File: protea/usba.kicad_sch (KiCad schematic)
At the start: 5 parts, among them J3 676430910, U7 USBLC6-2SC6

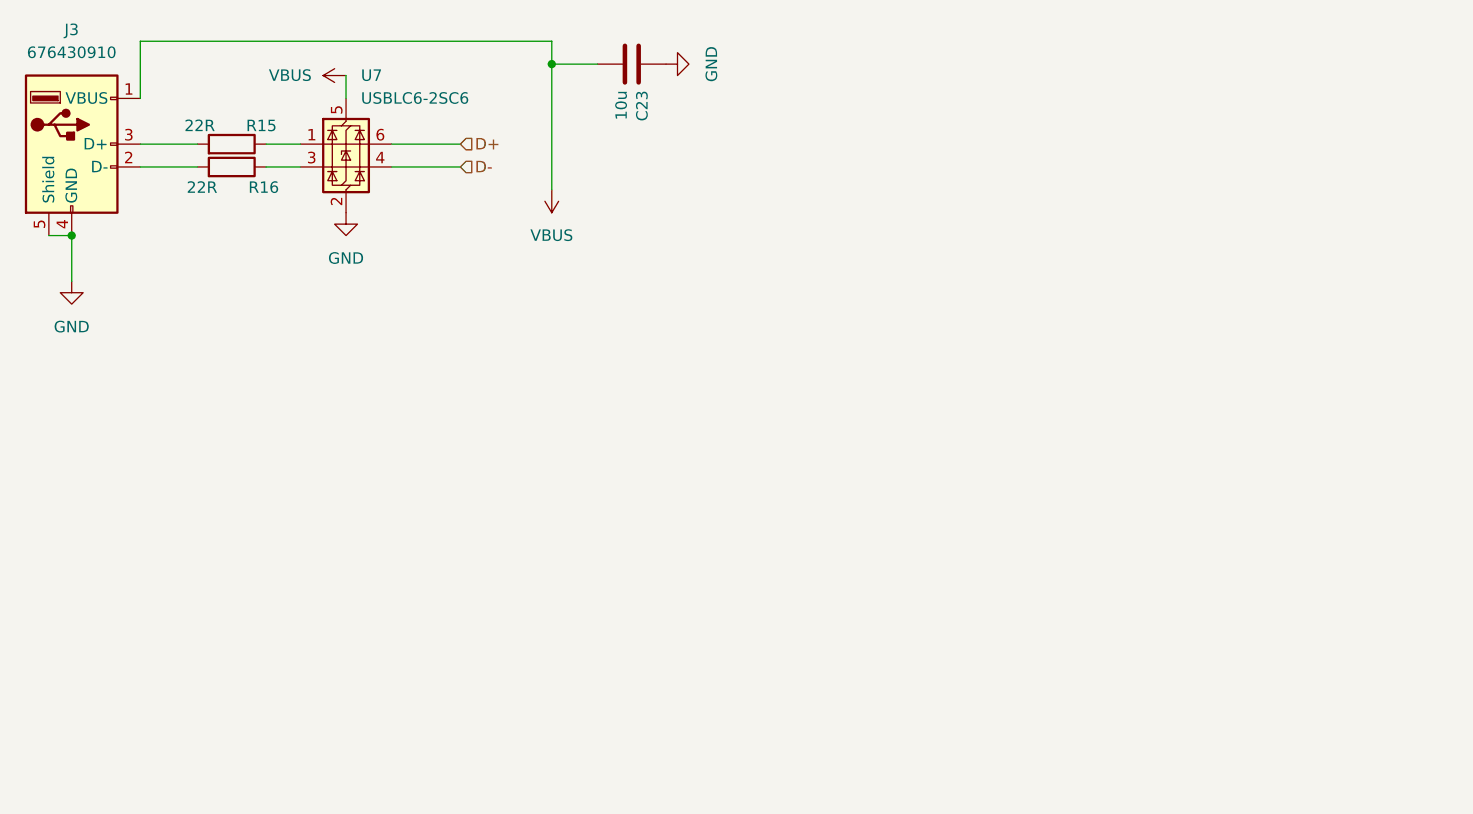
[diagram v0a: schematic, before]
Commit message: Protea HW 2.06
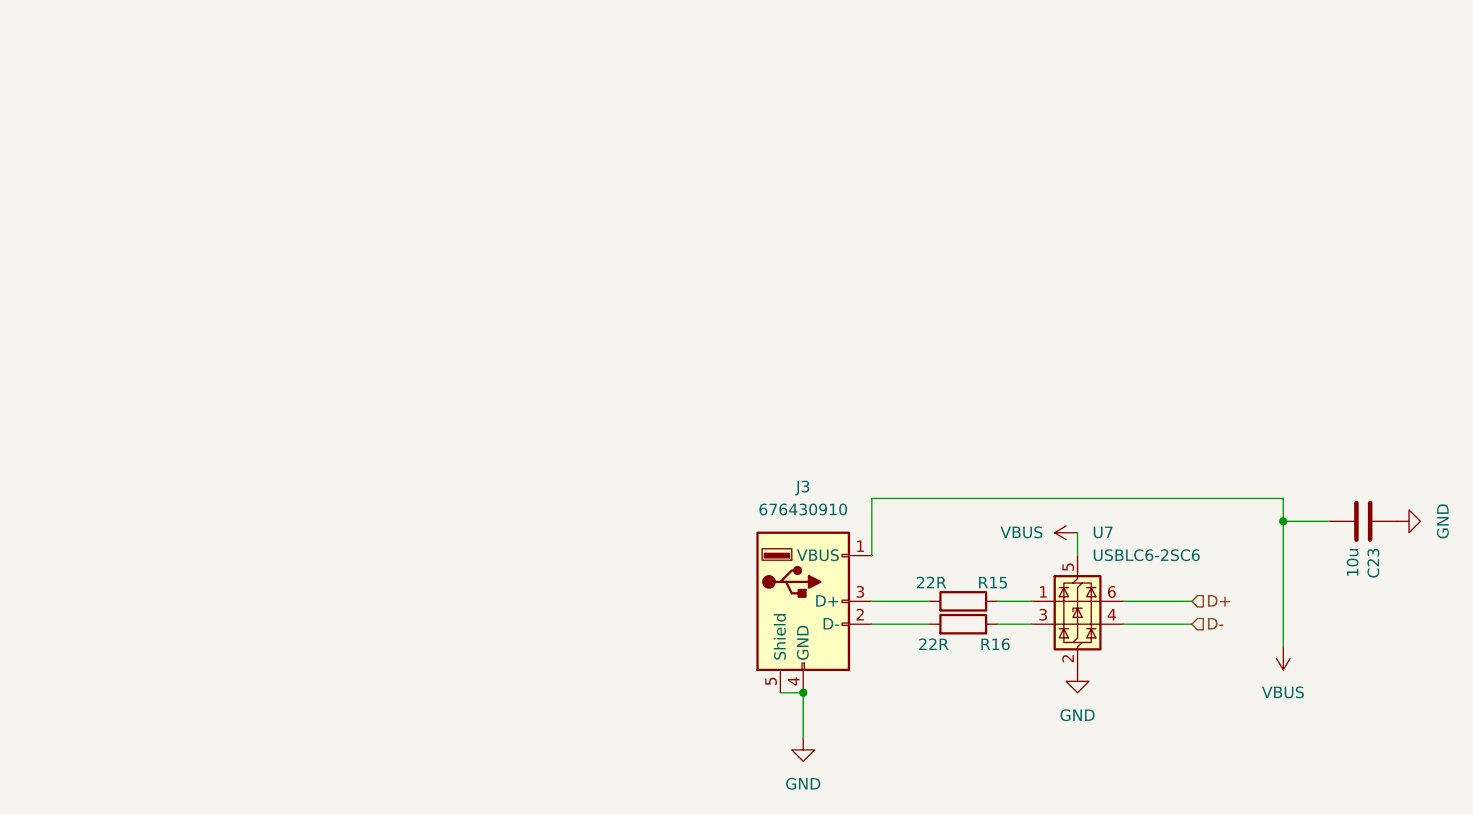
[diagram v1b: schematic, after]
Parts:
- J3: AliExpress (none) -> https://vi.aliexpress.com/item/32265708803.html
- U7: AliExpress (none) -> https://vi.aliexpress.com/item/1005006883533480.html
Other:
- moved on the sheet: C23, J3, R15, R16, U7
